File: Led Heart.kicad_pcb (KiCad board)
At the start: 2 copper layers, 30.5 x 27.2 mm, 47 parts, among them J1 Conn_01x01_Female, J2 Conn_01x01_Female, SW1 SW_DIP_x01, U1 STM32L031G6U6

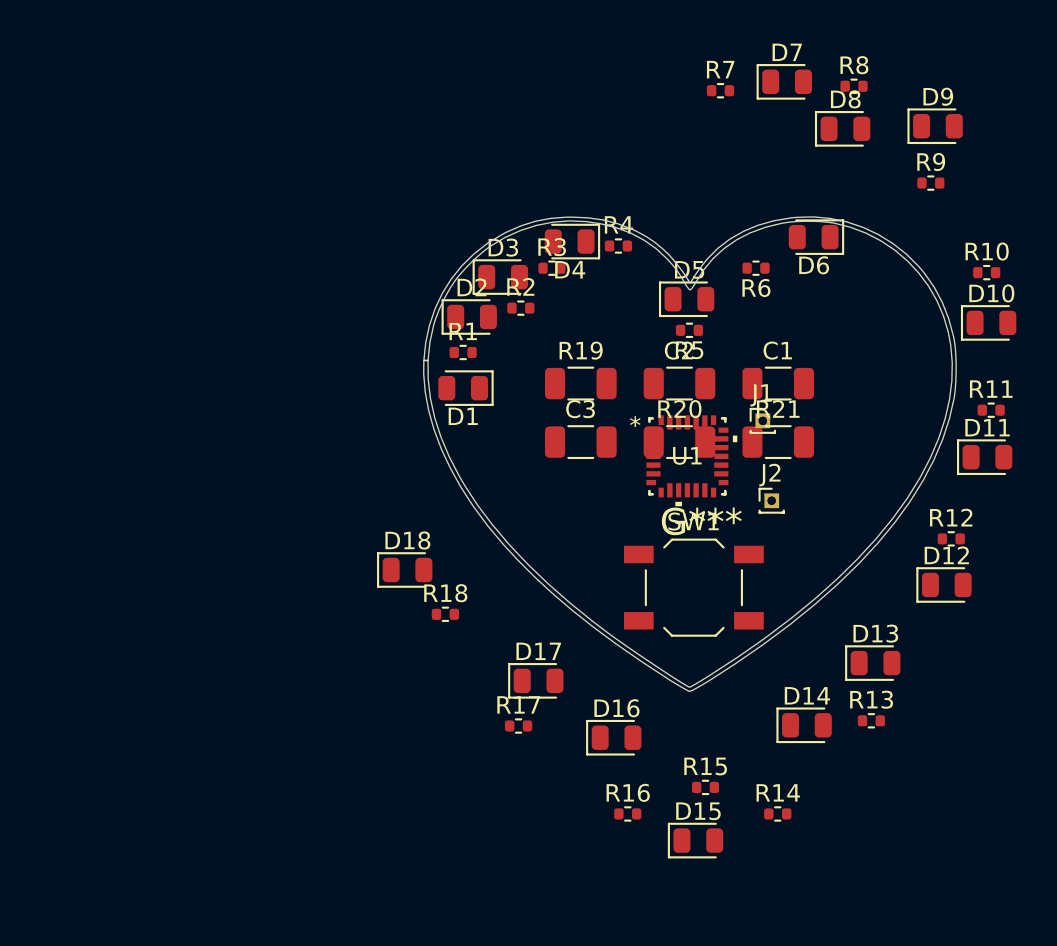
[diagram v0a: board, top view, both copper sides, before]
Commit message: Uporządkowanie pcb diody w trakcie podłączania
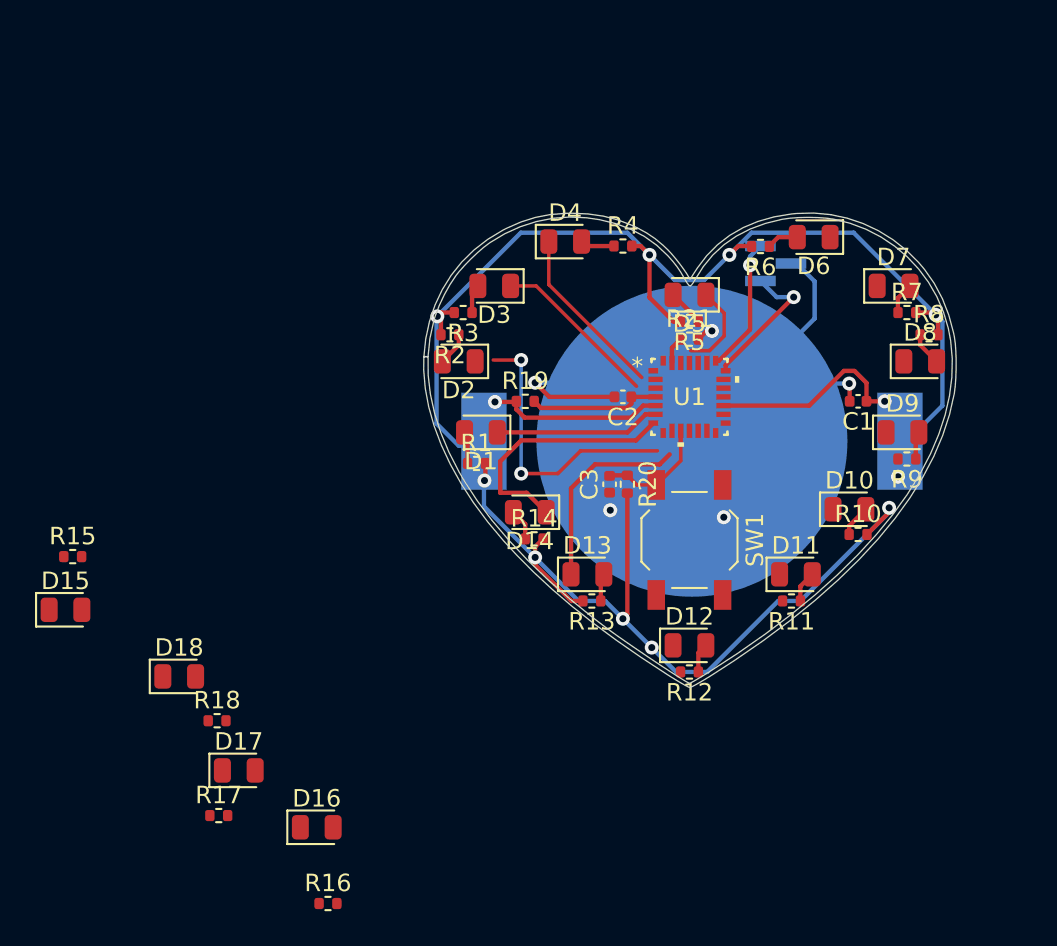
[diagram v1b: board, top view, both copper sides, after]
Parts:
- C1, C2, C3: footprint Capacitor_SMD:C_1206_3216Metric -> Capacitor_SMD:C_0402_1005Metric
- J1: value Conn_01x01_Female -> Conn_01x03_Female; footprint Connector_PinHeader_1.00mm:PinHeader_1x01_P1.00mm_Vertical -> Connector_PinHeader_1.00mm:PinHeader_1x03_P1.00mm_Vertical_SMD_Pin1Left; moved to B.Cu
- J2: value Conn_01x01_Female -> Conn_01x02_Female; footprint Connector_PinHeader_1.00mm:PinHeader_1x01_P1.00mm_Vertical -> Battery:BatteryHolder_MPD_BC2003_1x2032; moved to B.Cu
- R19, R20, R21: value 100k -> 10k; footprint Capacitor_SMD:C_1206_3216Metric -> Resistor_SMD:R_0402_1005Metric
- moved D15 38.6 mm to (71.2, 104.9)
- moved R15 38.6 mm to (71.6, 101.9)
- moved R14 21.0 mm to (98.0, 100.8)
- moved D14 20.0 mm to (97.8, 99.3), turned to 180 degrees
- moved D16 17.9 mm to (85.6, 117.3)
- moved D17 17.9 mm to (81.1, 114.1)
- moved R17 17.9 mm to (80.0, 116.7)
- moved R16 17.9 mm to (86.2, 121.7)
- moved D9 17.6 mm to (119.1, 94.7)
- moved R13 17.4 mm to (101.3, 104.4), turned to 180 degrees
- moved D13 17.3 mm to (101.1, 102.9)
- moved R12 16.8 mm to (106.9, 108.5), turned to 180 degrees
- moved R10 16.7 mm to (116.6, 100.6)
- moved R7 16.6 mm to (119.4, 87.9)
- moved R9 15.9 mm to (119.4, 96.3), turned to 180 degrees
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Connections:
- C3 pad 2: Net-(C3-Pad2) -> Net-(U1-Pad10)
- D14 pad 1: unconnected-(D14-Pad1) -> Net-(U1-Pad7)
- J2 pad 1: GND -> +3V0
- R20 pad 1: Net-(C3-Pad2) -> Net-(U1-Pad10)
- SW1 pad 2: Net-(C3-Pad2) -> Net-(U1-Pad10)
- U1 pad 10: unconnected-(U1-Pad10) -> Net-(U1-Pad10)
- U1 pad 21: Net-(U1-Pad21) -> Net-(J1-Pad1)
- U1 pad 22: Net-(U1-Pad22) -> Net-(J1-Pad3)
- U1 pad 7: unconnected-(U1-Pad7) -> Net-(U1-Pad7)
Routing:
- net +3V0: track 0.00 -> 144.7 mm, vias 0 -> 12
- net GND: track 0.00 -> 49.1 mm, vias 0 -> 5
- net (no net): track 0.00 -> 16.4 mm, vias 0 -> 2
- net Net-(U1-Pad7): track 0.00 -> 14.6 mm
- net unconnected-(D13-Pad1): track 0.00 -> 11.4 mm
- net unconnected-(D4-Pad1): track 0.00 -> 9.98 mm
- net unconnected-(D3-Pad1): track 0.00 -> 9.58 mm
- net Net-(D1-Pad1): track 0.00 -> 9.48 mm
- net Net-(J1-Pad1): track 0.00 -> 8.11 mm, vias 0 -> 1
- net Net-(C2-Pad1): track 0.00 -> 7.59 mm
- net Net-(U1-Pad10): track 0.00 -> 6.60 mm
- net unconnected-(D5-Pad1): track 0.00 -> 5.06 mm
- net Net-(D5-Pad2): track 0.00 -> 2.12 mm
- net Net-(D4-Pad2): track 0.00 -> 1.96 mm
- net Net-(D8-Pad2): track 0.00 -> 1.91 mm
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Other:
- outline, holes or cut-outs redrawn

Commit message: k
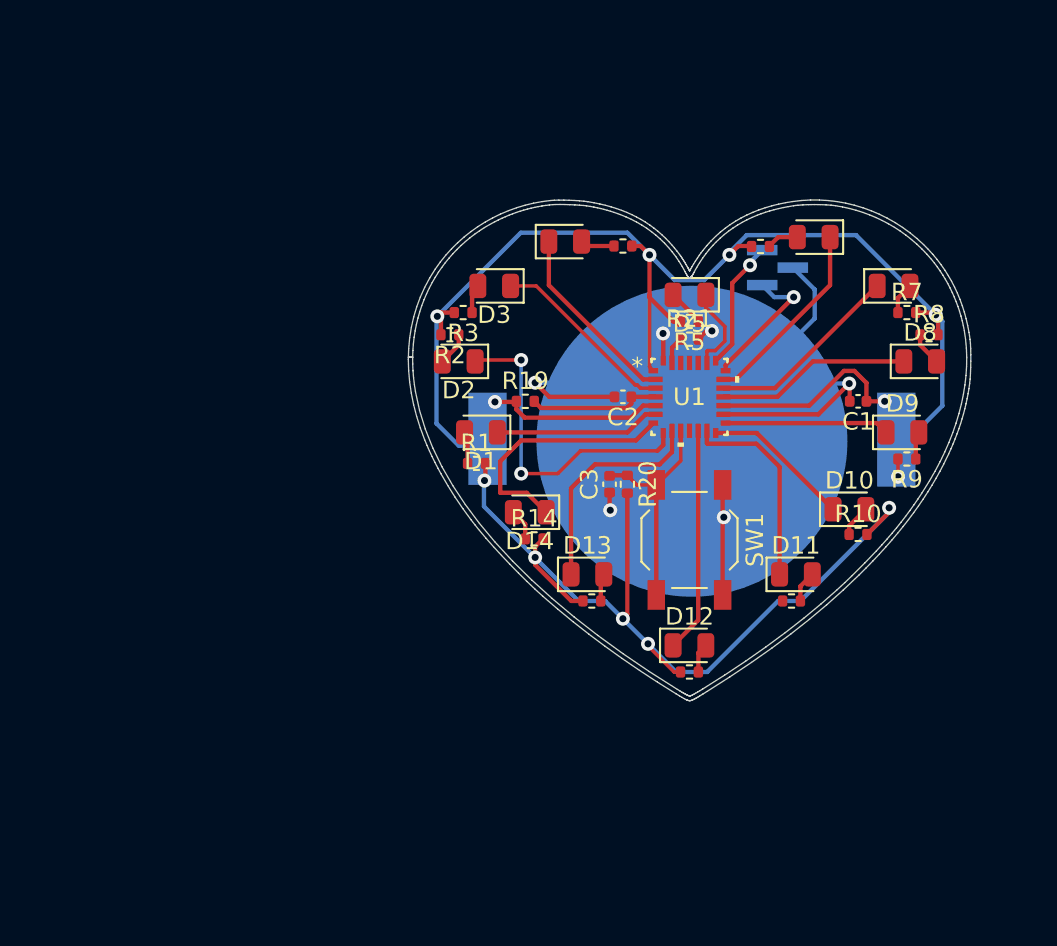
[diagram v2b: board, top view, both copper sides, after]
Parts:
- removed D15, D16, D17, D18: LED, Diode_SMD:D_0805_2012Metric
- removed G***: LOGO, LOGO
- removed R15, R16, R17, R18: 3.3k, Resistor_SMD:R_0402_1005Metric
- J2: footprint Battery:BatteryHolder_MPD_BC2003_1x2032 -> SamacSys_Parts:BatteryHolder_MPD_BC2003_1x2032
- moved J1 0.26 mm to (112.0, 85.3)
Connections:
- D10 pad 1: unconnected-(D10-Pad1) -> Net-(U1-Pad14)
- D11 pad 1: unconnected-(D11-Pad1) -> Net-(U1-Pad13)
- D12 pad 1: unconnected-(D12-Pad1) -> Net-(U1-Pad12)
- D13 pad 1: unconnected-(D13-Pad1) -> Net-(D13-Pad1)
- D2 pad 1: unconnected-(D2-Pad1) -> Net-(U1-Pad8)
- D3 pad 1: unconnected-(D3-Pad1) -> Net-(D3-Pad1)
- D4 pad 1: unconnected-(D4-Pad1) -> Net-(D4-Pad1)
- D5 pad 1: unconnected-(D5-Pad1) -> Net-(U1-Pad23)
- D6 pad 1: unconnected-(D6-Pad1) -> Net-(U1-Pad20)
- D7 pad 1: unconnected-(D7-Pad1) -> Net-(U1-Pad19)
- D8 pad 1: unconnected-(D8-Pad1) -> Net-(U1-Pad18)
- D9 pad 1: unconnected-(D9-Pad1) -> Net-(U1-Pad15)
- U1 pad 12: unconnected-(U1-Pad12) -> Net-(U1-Pad12)
- U1 pad 13: unconnected-(U1-Pad13) -> Net-(U1-Pad13)
- U1 pad 14: unconnected-(U1-Pad14) -> Net-(U1-Pad14)
- U1 pad 15: unconnected-(U1-Pad15) -> Net-(U1-Pad15)
- U1 pad 18: unconnected-(U1-Pad18) -> Net-(U1-Pad18)
- U1 pad 19: unconnected-(U1-Pad19) -> Net-(U1-Pad19)
- U1 pad 2: unconnected-(U1-Pad2) -> Net-(D4-Pad1)
- U1 pad 20: unconnected-(U1-Pad20) -> Net-(U1-Pad20)
- U1 pad 23: unconnected-(U1-Pad23) -> Net-(U1-Pad23)
- U1 pad 3: unconnected-(U1-Pad3) -> Net-(D3-Pad1)
- U1 pad 8: unconnected-(U1-Pad8) -> Net-(U1-Pad8)
- U1 pad 9: unconnected-(U1-Pad9) -> Net-(D13-Pad1)
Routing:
- net Net-(U1-Pad8): track 0.00 -> 18.7 mm, vias 0 -> 2
- net (no net): track 16.4 -> 0.00 mm, vias 2 -> 0
- net GND: track 49.1 -> 65.5 mm, vias 5 -> 6
- net Net-(U1-Pad12): track 0.00 -> 12.9 mm
- net Net-(D13-Pad1): track 0.00 -> 12.8 mm
- net Net-(U1-Pad13): track 0.00 -> 11.6 mm
- net unconnected-(D13-Pad1): track 11.4 -> 0.00 mm
- net Net-(U1-Pad19): track 0.00 -> 11.2 mm
- net Net-(U1-Pad18): track 0.00 -> 11.2 mm
- net Net-(U1-Pad20): track 0.00 -> 11.1 mm
- net Net-(D4-Pad1): track 0.00 -> 10.8 mm
- net Net-(D3-Pad1): track 0.00 -> 10.7 mm
- net unconnected-(D4-Pad1): track 9.98 -> 0.00 mm
- net unconnected-(D3-Pad1): track 9.58 -> 0.00 mm
- net Net-(U1-Pad15): track 0.00 -> 9.40 mm
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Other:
- board size 30.5 x 27.2 mm -> 32.2 x 28.7 mm
